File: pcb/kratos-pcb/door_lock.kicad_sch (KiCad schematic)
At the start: 6 parts, among them Q2 2N2222A, Q3 2N2222A

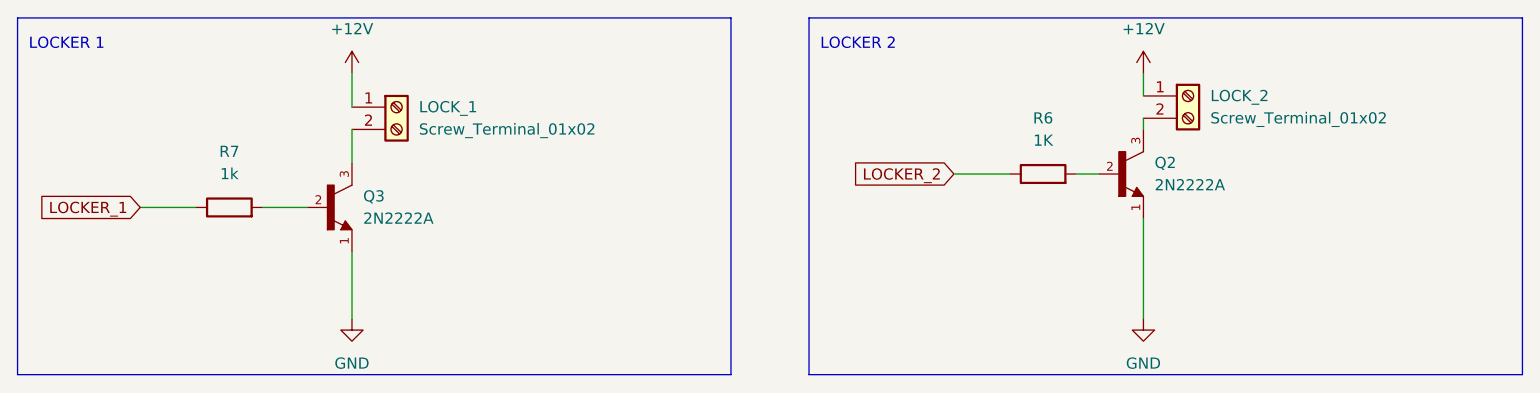
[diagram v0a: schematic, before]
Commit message: ## updatee
- gitignor
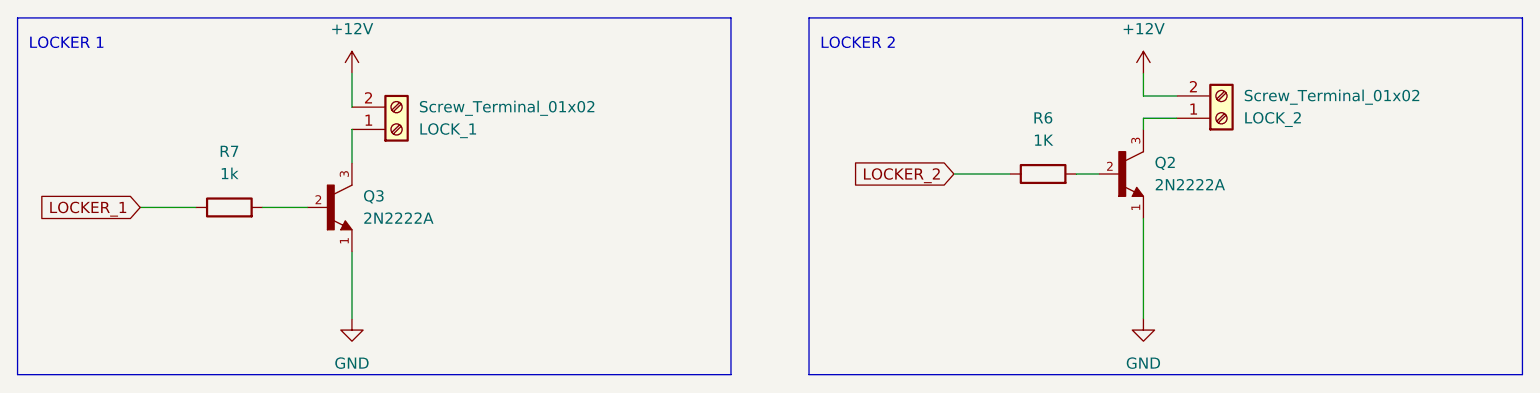
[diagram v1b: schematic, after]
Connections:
- net +12V: now also LOCK_1.2 (Pin_2), LOCK_2.2 (Pin_2); no longer LOCK_1.1 (Pin_1), LOCK_2.1 (Pin_1)
- net at Q3.3: now also LOCK_1.1 (Pin_1); no longer LOCK_1.2 (Pin_2)
- net at Q2.3: now also LOCK_2.1 (Pin_1); no longer LOCK_2.2 (Pin_2)
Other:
- moved on the sheet: LOCK_2
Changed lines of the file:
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@@
 (kicad_sch (version 20230121) (generator eeschema)
   (paper "A4")
-  (wire (pts (xy 185.42 62.23) (xy 185.42 64.77))
-    (stroke (width 0) (type default))
-  )
   (wire (pts (xy 185.42 67.31) (xy 185.42 68.58))
     (stroke (width 0) (type default))
@@
     (stroke (width 0) (type default))
   )
+  (wire (pts (xy 189.23 67.31) (xy 185.42 67.31))
+    (stroke (width 0) (type default))
+  )
   (wire (pts (xy 163.83 73.66) (xy 170.18 73.66))
     (stroke (width 0) (type default))
@@
   )
   (wire (pts (xy 71.12 77.47) (xy 77.47 77.47))
+    (stroke (width 0) (type default))
+  )
+  (wire (pts (xy 189.23 64.77) (xy 185.42 64.77))
+    (stroke (width 0) (type default))
+  )
+  (wire (pts (xy 185.42 64.77) (xy 185.42 62.23))
     (stroke (width 0) (type default))
   )
@@
     )
   )
-  (symbol (lib_id "Connector:Screw_Terminal_01x02") (at 190.5 64.77 0) (unit 1)
+  (symbol (lib_id "Connector:Screw_Terminal_01x02") (at 194.31 67.31 0) (mirror x) (unit 1)
     (in_bom yes) (on_board yes) (dnp no)
-    (property "Reference" "LOCK_2" (at 193.04 64.77 0)
-      (effects (font (size 1.27 1.27)) (justify left))
-    )
-    (property "Value" "Screw_Terminal_01x02" (at 193.04 67.31 0)
-      (effects (font (size 1.27 1.27)) (justify left))
-    )
-    (property "Footprint" "TerminalBlock:TerminalBlock_bornier-2_P5.08mm" (at 190.5 64.77 0)
-      (effects (font (size 1.27 1.27)) hide)
-    )
-    (property "Datasheet" "~" (at 190.5 64.77 0)
+    (property "Reference" "LOCK_2" (at 196.85 67.31 0)
+      (effects (font (size 1.27 1.27)) (justify left))
+    )
+    (property "Value" "Screw_Terminal_01x02" (at 196.85 64.77 0)
+      (effects (font (size 1.27 1.27)) (justify left))
+    )
+    (property "Footprint" "TerminalBlock:TerminalBlock_bornier-2_P5.08mm" (at 194.31 67.31 0)
+      (effects (font (size 1.27 1.27)) hide)
+    )
+    (property "Datasheet" "~" (at 194.31 67.31 0)
       (effects (font (size 1.27 1.27)) hide)
     )
@@
     )
   )
-  (symbol (lib_id "Connector:Screw_Terminal_01x02") (at 100.33 66.04 0) (unit 1)
+  (symbol (lib_id "Connector:Screw_Terminal_01x02") (at 100.33 68.58 0) (mirror x) (unit 1)
     (in_bom yes) (on_board yes) (dnp no)
-    (property "Reference" "LOCK_1" (at 102.87 66.04 0)
-      (effects (font (size 1.27 1.27)) (justify left))
-    )
-    (property "Value" "Screw_Terminal_01x02" (at 102.87 68.58 0)
-      (effects (font (size 1.27 1.27)) (justify left))
-    )
-    (property "Footprint" "TerminalBlock:TerminalBlock_bornier-2_P5.08mm" (at 100.33 66.04 0)
-      (effects (font (size 1.27 1.27)) hide)
-    )
-    (property "Datasheet" "~" (at 100.33 66.04 0)
-      (effects (font (size 1.27 1.27)) hide)
-    )
+    (property "Reference" "LOCK_1" (at 102.87 68.58 0)
+      (effects (font (size 1.27 1.27)) (justify left))
+    )
+    (property "Value" "Screw_Terminal_01x02" (at 102.87 66.04 0)
+      (effects (font (size 1.27 1.27)) (justify left))
+    )
+    (property "Footprint" "TerminalBlock:TerminalBlock_bornier-2_P5.08mm" (at 100.33 68.58 0)
+      (effects (font (size 1.27 1.27)) hide)
+    )
+    (property "Datasheet" "~" (at 100.33 68.58 0)
+      (effects (font (size 1.27 1.27)) hide)
+    )

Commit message: ### added
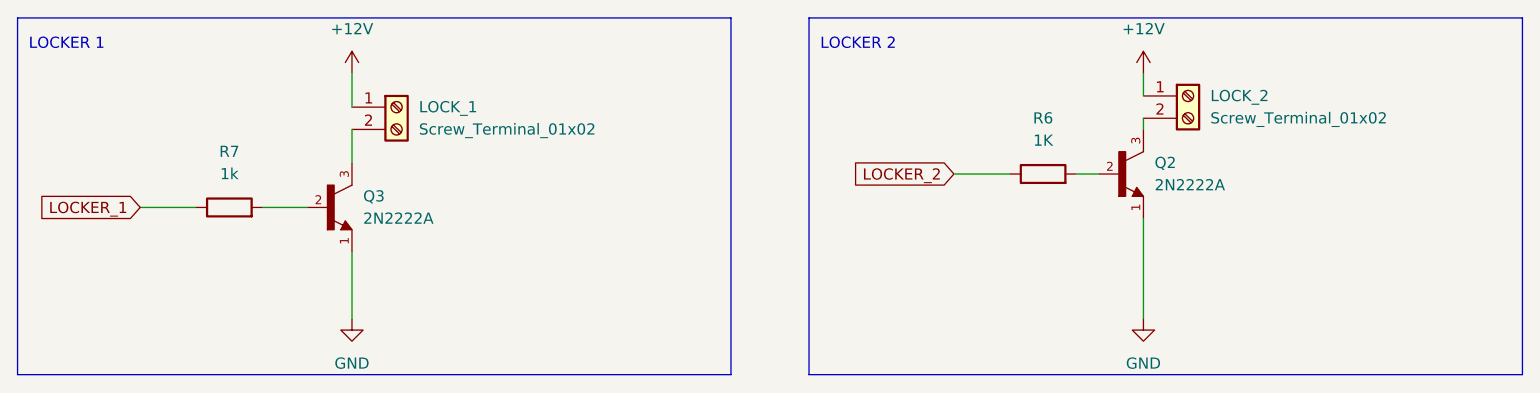
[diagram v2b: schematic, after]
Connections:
- net +12V: now also LOCK_1.1 (Pin_1), LOCK_2.1 (Pin_1); no longer LOCK_1.2 (Pin_2), LOCK_2.2 (Pin_2)
- net at Q3.3: now also LOCK_1.2 (Pin_2); no longer LOCK_1.1 (Pin_1)
- net at Q2.3: now also LOCK_2.2 (Pin_2); no longer LOCK_2.1 (Pin_1)
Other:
- moved on the sheet: LOCK_2
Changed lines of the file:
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@@
 (kicad_sch (version 20230121) (generator eeschema)
   (paper "A4")
+  (wire (pts (xy 185.42 62.23) (xy 185.42 64.77))
+    (stroke (width 0) (type default))
+  )
   (wire (pts (xy 185.42 67.31) (xy 185.42 68.58))
     (stroke (width 0) (type default))
@@
     (stroke (width 0) (type default))
   )
-  (wire (pts (xy 189.23 67.31) (xy 185.42 67.31))
-    (stroke (width 0) (type default))
-  )
   (wire (pts (xy 163.83 73.66) (xy 170.18 73.66))
     (stroke (width 0) (type default))
@@
   )
   (wire (pts (xy 71.12 77.47) (xy 77.47 77.47))
-    (stroke (width 0) (type default))
-  )
-  (wire (pts (xy 189.23 64.77) (xy 185.42 64.77))
-    (stroke (width 0) (type default))
-  )
-  (wire (pts (xy 185.42 64.77) (xy 185.42 62.23))
     (stroke (width 0) (type default))
   )
@@
     )
   )
-  (symbol (lib_id "Connector:Screw_Terminal_01x02") (at 194.31 67.31 0) (mirror x) (unit 1)
+  (symbol (lib_id "Connector:Screw_Terminal_01x02") (at 190.5 64.77 0) (unit 1)
     (in_bom yes) (on_board yes) (dnp no)
-    (property "Reference" "LOCK_2" (at 196.85 67.31 0)
-      (effects (font (size 1.27 1.27)) (justify left))
-    )
-    (property "Value" "Screw_Terminal_01x02" (at 196.85 64.77 0)
-      (effects (font (size 1.27 1.27)) (justify left))
-    )
-    (property "Footprint" "TerminalBlock:TerminalBlock_bornier-2_P5.08mm" (at 194.31 67.31 0)
-      (effects (font (size 1.27 1.27)) hide)
-    )
-    (property "Datasheet" "~" (at 194.31 67.31 0)
+    (property "Reference" "LOCK_2" (at 193.04 64.77 0)
+      (effects (font (size 1.27 1.27)) (justify left))
+    )
+    (property "Value" "Screw_Terminal_01x02" (at 193.04 67.31 0)
+      (effects (font (size 1.27 1.27)) (justify left))
+    )
+    (property "Footprint" "TerminalBlock:TerminalBlock_bornier-2_P5.08mm" (at 190.5 64.77 0)
+      (effects (font (size 1.27 1.27)) hide)
+    )
+    (property "Datasheet" "~" (at 190.5 64.77 0)
       (effects (font (size 1.27 1.27)) hide)
     )
@@
     )
   )
-  (symbol (lib_id "Connector:Screw_Terminal_01x02") (at 100.33 68.58 0) (mirror x) (unit 1)
+  (symbol (lib_id "Connector:Screw_Terminal_01x02") (at 100.33 66.04 0) (unit 1)
     (in_bom yes) (on_board yes) (dnp no)
-    (property "Reference" "LOCK_1" (at 102.87 68.58 0)
-      (effects (font (size 1.27 1.27)) (justify left))
-    )
-    (property "Value" "Screw_Terminal_01x02" (at 102.87 66.04 0)
-      (effects (font (size 1.27 1.27)) (justify left))
-    )
-    (property "Footprint" "TerminalBlock:TerminalBlock_bornier-2_P5.08mm" (at 100.33 68.58 0)
-      (effects (font (size 1.27 1.27)) hide)
-    )
-    (property "Datasheet" "~" (at 100.33 68.58 0)
-      (effects (font (size 1.27 1.27)) hide)
-    )
+    (property "Reference" "LOCK_1" (at 102.87 66.04 0)
+      (effects (font (size 1.27 1.27)) (justify left))
+    )
+    (property "Value" "Screw_Terminal_01x02" (at 102.87 68.58 0)
+      (effects (font (size 1.27 1.27)) (justify left))
+    )
+    (property "Footprint" "TerminalBlock:TerminalBlock_bornier-2_P5.08mm" (at 100.33 66.04 0)
+      (effects (font (size 1.27 1.27)) hide)
+    )
+    (property "Datasheet" "~" (at 100.33 66.04 0)
+      (effects (font (size 1.27 1.27)) hide)
+    )
